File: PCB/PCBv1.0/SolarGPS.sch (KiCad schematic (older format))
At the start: 56 parts, among them J1 Conn_01x10_Female, J2 Solar1+, J3 GND, J4 Conn_02x05_Odd_Even, J5 Solar2+, J6 GND, J7 Screw_Terminal_01x01, U2 MAX-M10Q, U4 STM32WB5MMGH6TR, U5 BQ25505, U6 LIS3DH, U7 TPS63802

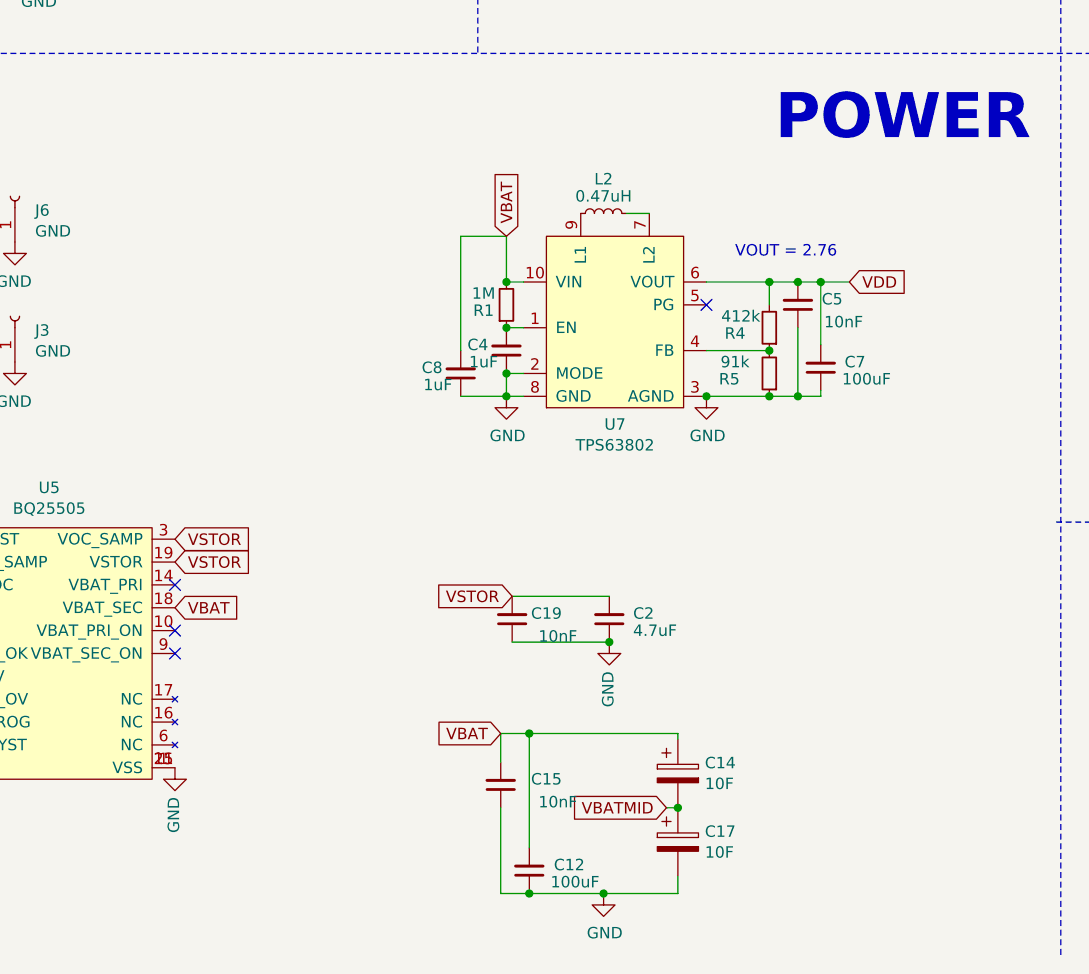
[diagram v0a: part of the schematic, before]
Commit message: Most Cost Savings
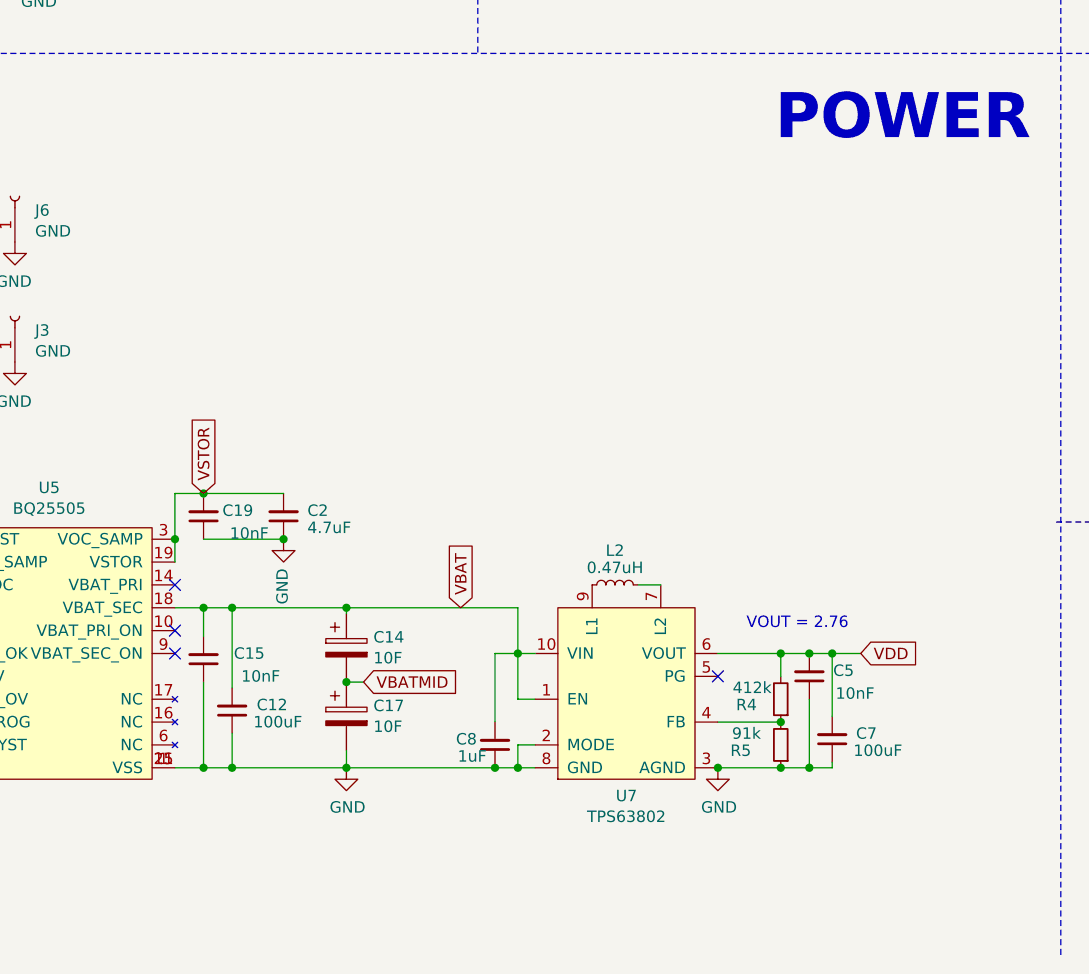
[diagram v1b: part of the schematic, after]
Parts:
- removed C4: 1uF, Capacitor_SMD:C_0603_1608Metric, symbol Device:C_Small
- removed R1: 1M, Resistor_SMD:R_0603_1608Metric, symbol Device:R_Small
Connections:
- net VBAT: now also U7.1 (EN)
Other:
- moved on the sheet: C12, C14, C15, C17, C19, C2, C5, C7, C8, L2, R4, R5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
